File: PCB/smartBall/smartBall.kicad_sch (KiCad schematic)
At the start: 9 parts, among them IC12 ADM7155ACPZ-04-R7, IC3 ESP32-S3-WROOM-1-N4R8

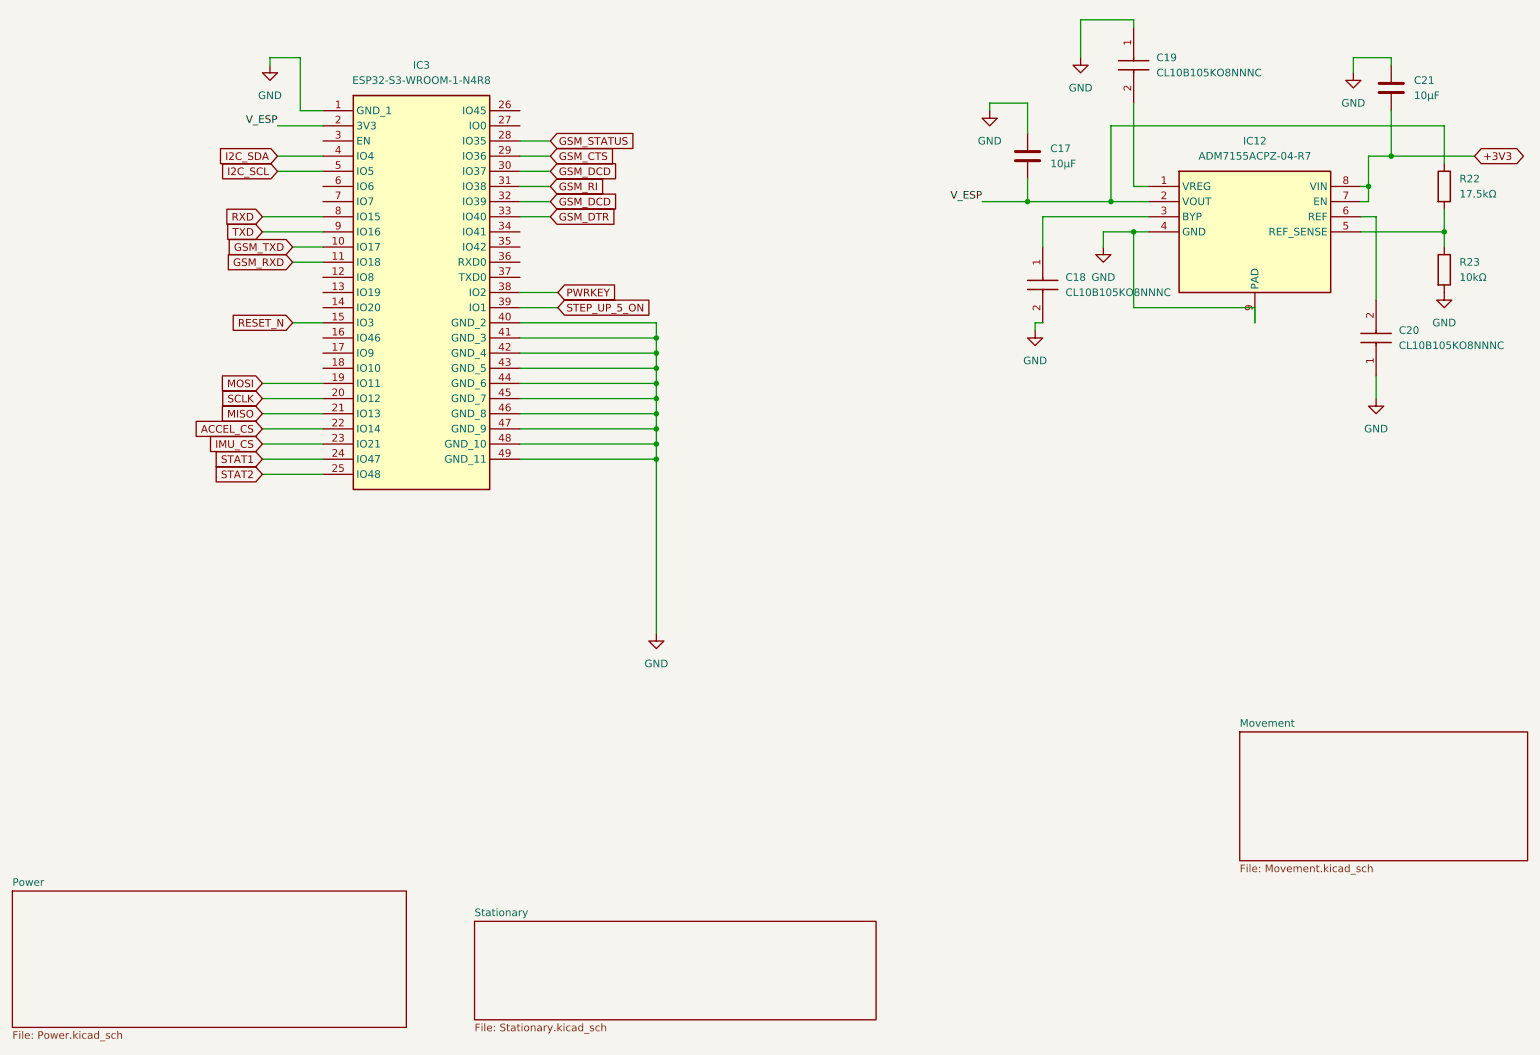
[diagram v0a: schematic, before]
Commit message: schematic ready
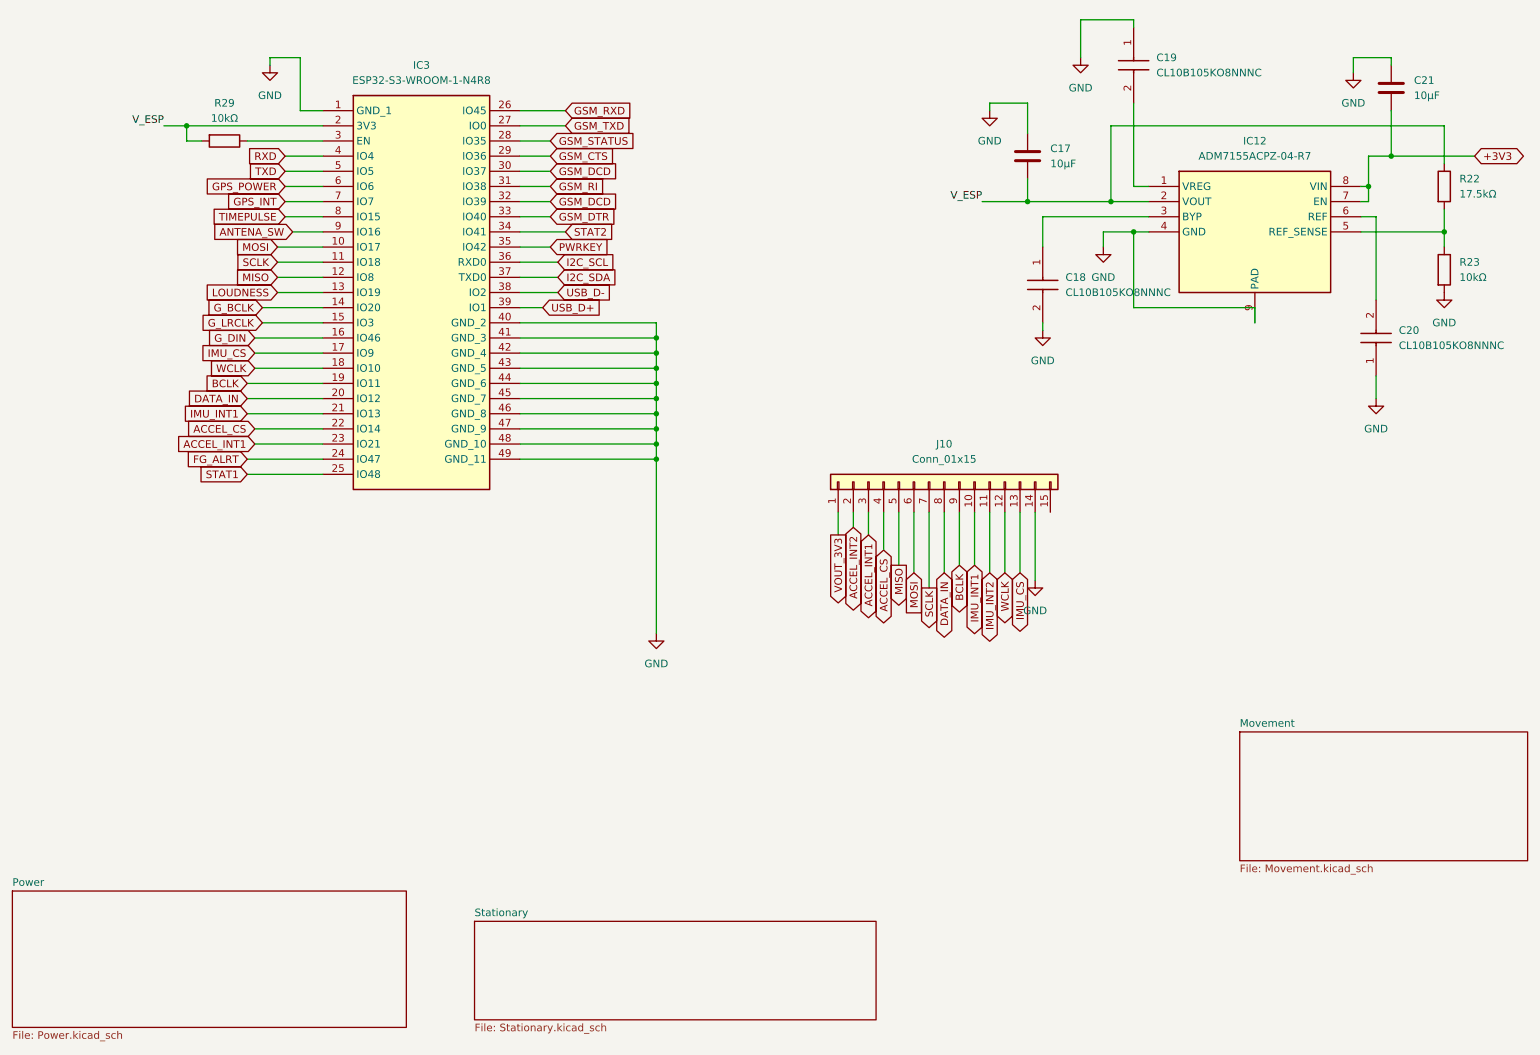
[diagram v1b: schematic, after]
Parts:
- added J10: Conn_01x15, symbol Connector_Generic:Conn_01x15
- added R29: 10kΩ, symbol Device:R
- IC12: footprint SON50P300X300X80-9N-D -> ADM7155ACPZ-04-07:SON50P300X300X80-9N-D
- IC3: footprint ESP32S3WROOM1N4R8 -> ESP_32-S3-WROOM-1-N4R8:ESP32S3WROOM1N4R8
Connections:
- net ACCEL_CS: now also J10.4 (Pin_4)
- net GND: now also J10.14 (Pin_14)
- net GSM_RXD: now also IC3.26 (IO45); no longer IC3.11 (IO18)
- net GSM_TXD: now also IC3.27 (IO0); no longer IC3.10 (IO17)
- net I2C_SCL: now also IC3.36 (RXD0); no longer IC3.5 (IO5)
- net I2C_SDA: now also IC3.37 (TXD0); no longer IC3.4 (IO4)
- net IMU_CS: now also IC3.17 (IO9), J10.13 (Pin_13); no longer IC3.23 (IO21)
- net MISO: now also IC3.12 (IO8), J10.5 (Pin_5); no longer IC3.21 (IO13)
- net MOSI: now also IC3.10 (IO17), J10.6 (Pin_6); no longer IC3.19 (IO11)
- net PWRKEY: now also IC3.35 (IO42); no longer IC3.38 (IO2)
- net RXD: now also IC3.4 (IO4); no longer IC3.8 (IO15)
- net SCLK: now also IC3.11 (IO18), J10.7 (Pin_7); no longer IC3.20 (IO12)
- net STAT1: now also IC3.25 (IO48); no longer IC3.24 (IO47)
- net STAT2: now also IC3.34 (IO41); no longer IC3.25 (IO48)
- net TXD: now also IC3.5 (IO5); no longer IC3.9 (IO16)
- net V_ESP: now also R29.2
- net LOUDNESS: now reaches IC3.13 (IO19)
- net G_BCLK: now reaches IC3.14 (IO20)
- net G_DIN: now reaches IC3.16 (IO46)
- net WCLK: now reaches IC3.18 (IO10)
- net WCLK: now also J10.12 (Pin_12)
- net at IC3.3 (EN): now also R29.1
- net GPS_POWER: now reaches IC3.6 (IO6)
- net GPS_INT: now reaches IC3.7 (IO7)
- net RESET_N renamed G_LRCLK
- net STEP_UP_5_ON renamed USB_D+
- new net ACCEL_INT1: IC3.23 (IO21), J10.3 (Pin_3)
- new net ACCEL_INT2: J10.2 (Pin_2)
- new net ANTENA_SW: IC3.9 (IO16)
- new net BCLK: IC3.19 (IO11), J10.9 (Pin_9)
- new net DATA_IN: IC3.20 (IO12), J10.8 (Pin_8)
- new net FG_ALRT: IC3.24 (IO47)
- new net IMU_INT1: IC3.21 (IO13), J10.10 (Pin_10)
- new net IMU_INT2: J10.11 (Pin_11)
- new net TIMEPULSE: IC3.8 (IO15)
- new net USB_D-: IC3.38 (IO2)
- new net VOUT_3V3: J10.1 (Pin_1)

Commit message: footprints assigned
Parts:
- C17, C21: footprint (none) -> Capacitor_THT:CP_Radial_Tantal_D5.0mm_P2.50mm
- C18, C19, C20: footprint CAPC1608X90N -> CL10B105KO8NNNC:CAPC1608X90N
- J10: footprint (none) -> Connector_PinHeader_2.54mm:PinHeader_1x15_P2.54mm_Vertical
- R22, R23, R29: footprint (none) -> Resistor_THT:R_Axial_DIN0207_L6.3mm_D2.5mm_P7.62mm_Horizontal
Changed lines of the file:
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@@
 			)
 		)
-		(property "Footprint" "CAPC1608X90N"
+		(property "Footprint" "CL10B105KO8NNNC:CAPC1608X90N"
 			(at 343.84 68.58 0)
 			(effects
@@
 			)
 		)
-		(property "Footprint" ""
+		(property "Footprint" "Resistor_THT:R_Axial_DIN0207_L6.3mm_D2.5mm_P7.62mm_Horizontal"
 			(at 257.302 59.69 90)
 			(effects
@@
 			)
 		)
-		(property "Footprint" ""
+		(property "Footprint" "Capacitor_THT:CP_Radial_Tantal_D5.0mm_P2.50mm"
 			(at 251.1552 33.02 0)
 			(effects
@@
 			)
 		)
-		(property "Footprint" "CAPC1608X90N"
+		(property "Footprint" "CL10B105KO8NNNC:CAPC1608X90N"
 			(at 95.58 64.77 0)
 			(effects
@@
 			)
 		)
-		(property "Footprint" ""
+		(property "Footprint" "Resistor_THT:R_Axial_DIN0207_L6.3mm_D2.5mm_P7.62mm_Horizontal"
 			(at 257.302 45.72 90)
 			(effects
@@
 			)
 		)
-		(property "Footprint" ""
+		(property "Footprint" "Connector_PinHeader_2.54mm:PinHeader_1x15_P2.54mm_Vertical"
 			(at 175.26 95.25 0)
 			(effects
@@
 			)
 		)
-		(property "Footprint" ""
+		(property "Footprint" "Capacitor_THT:CP_Radial_Tantal_D5.0mm_P2.50mm"
 			(at 190.1952 44.45 0)
 			(effects
@@
 			)
 		)
-		(property "Footprint" "CAPC1608X90N"
+		(property "Footprint" "CL10B105KO8NNNC:CAPC1608X90N"
 			(at 110.82 27.94 0)
 			(effects
@@
 			)
 		)
-		(property "Footprint" ""
+		(property "Footprint" "Resistor_THT:R_Axial_DIN0207_L6.3mm_D2.5mm_P7.62mm_Horizontal"
 			(at 54.61 36.322 90)
 			(effects

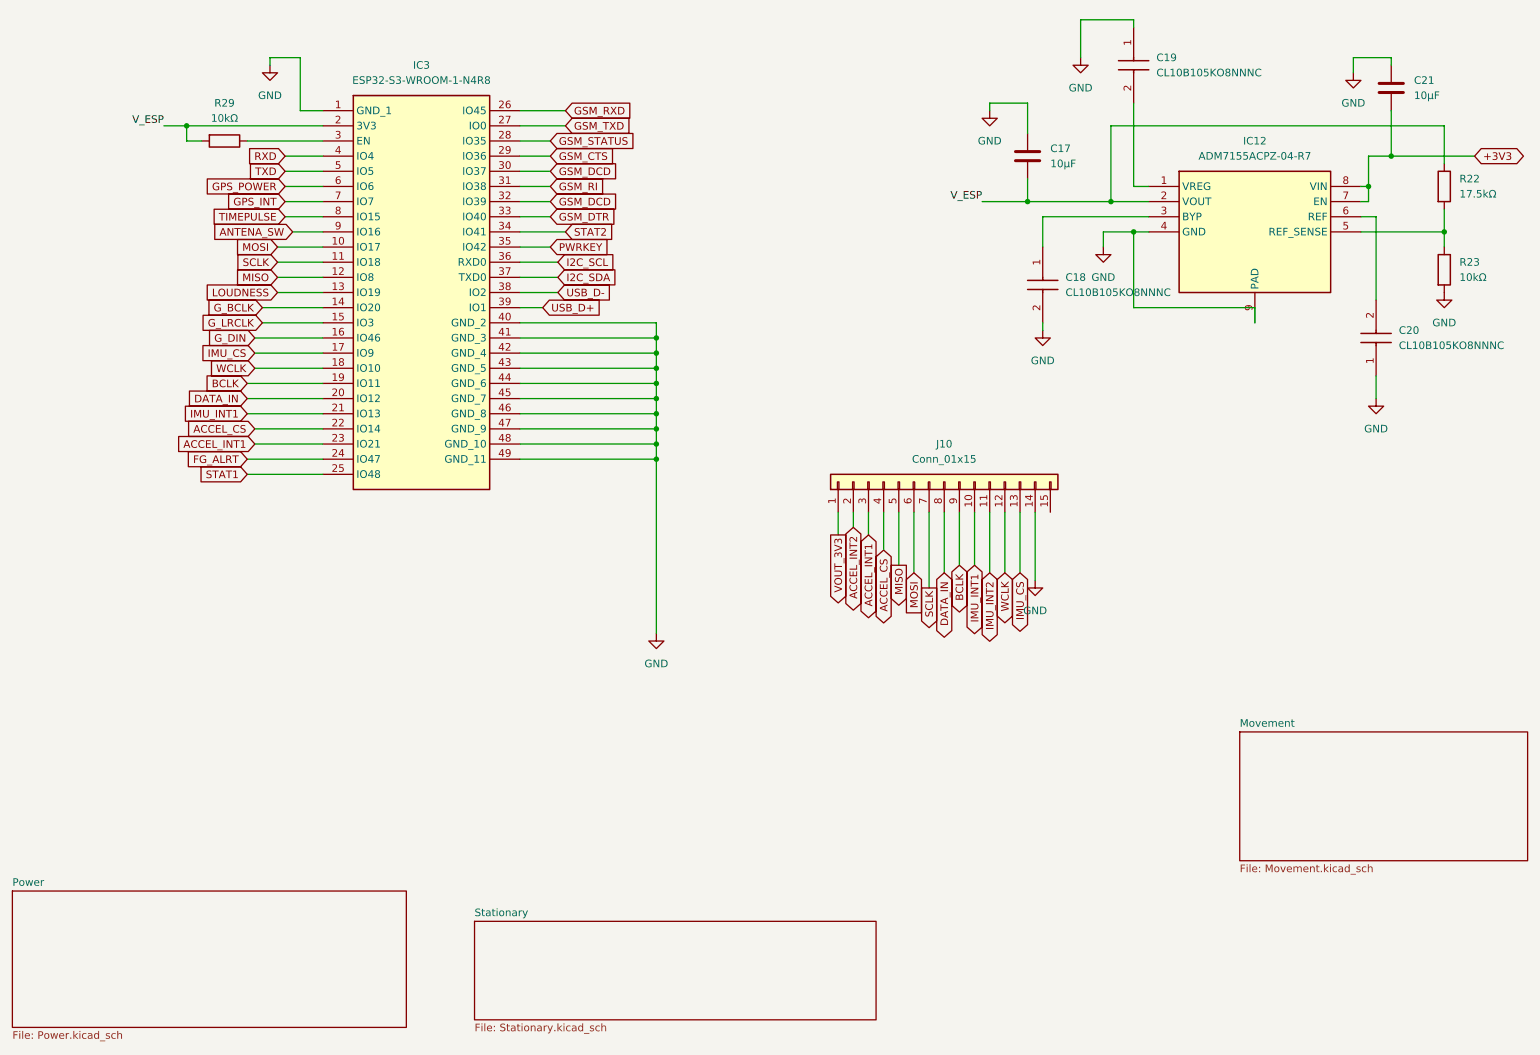
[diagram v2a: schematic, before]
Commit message: updated to hierarchical labels
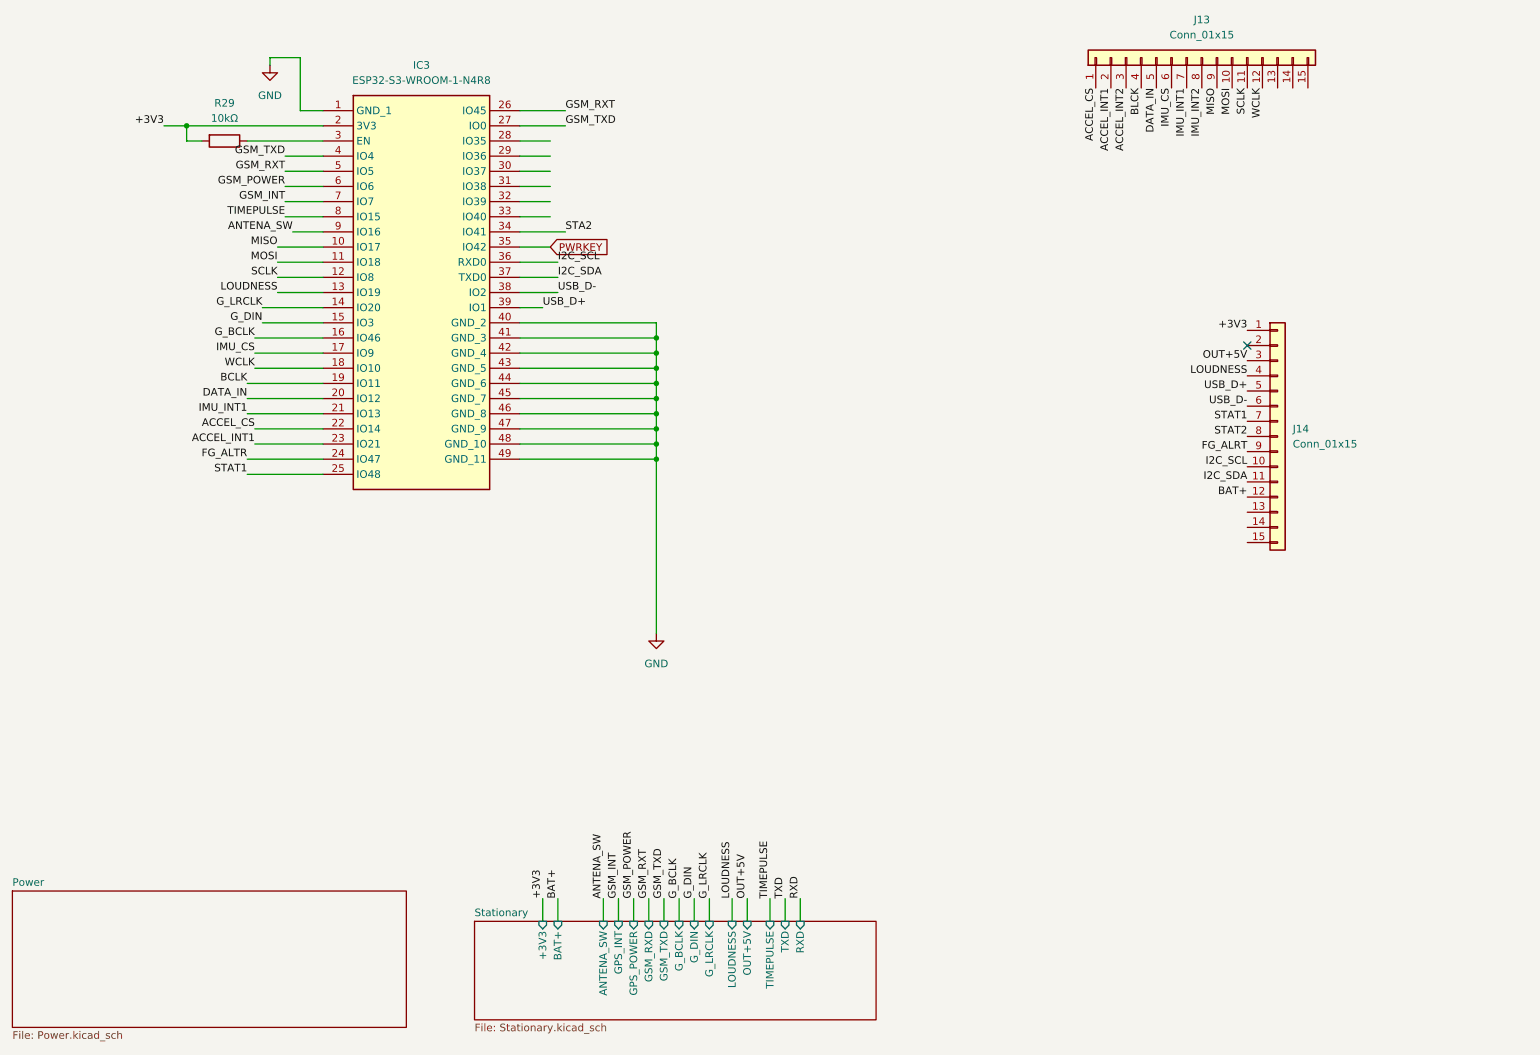
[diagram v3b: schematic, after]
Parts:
- removed C17, C21: 10µF, Capacitor_THT:CP_Radial_Tantal_D5.0mm_P2.50mm, symbol Device:C
- removed C18, C19, C20: CL10B105KO8NNNC, CL10B105KO8NNNC:CAPC1608X90N, symbol CL10B105KO8NNNC:CL10B105KO8NNNC
- removed IC12: ADM7155ACPZ-04-R7, ADM7155ACPZ-04-07:SON50P300X300X80-9N-D, symbol ADM7155ACPZ-04-R7:ADM7155ACPZ-04-R7
- removed J10: Conn_01x15, Connector_PinHeader_2.54mm:PinHeader_1x15_P2.54mm_Vertical, symbol Connector_Generic:Conn_01x15
- removed R22: 17.5kΩ, Resistor_THT:R_Axial_DIN0207_L6.3mm_D2.5mm_P7.62mm_Horizontal, symbol Device:R
- removed R23: 10kΩ, Resistor_THT:R_Axial_DIN0207_L6.3mm_D2.5mm_P7.62mm_Horizontal, symbol Device:R
- added J13, J14: Conn_01x15, Connector_PinHeader_2.54mm:PinHeader_1x15_P2.54mm_Vertical, symbol Connector_Generic:Conn_01x15
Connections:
- net V_ESP is gone; now on net +3V3: IC3.2 (3V3), R29.2
- net +3V3: now also J14.1 (Pin_1)
- net ACCEL_CS: now also J13.1 (Pin_1)
- net ACCEL_INT1: now also J13.2 (Pin_2)
- net ACCEL_INT2: now also J13.3 (Pin_3)
- net DATA_IN: now also J13.5 (Pin_5)
- net FG_ALRT: now also J14.9 (Pin_9); no longer IC3.24 (IO47)
- net GSM_TXD: now also IC3.4 (IO4)
- net G_BCLK: now also IC3.16 (IO46); no longer IC3.14 (IO20)
- net G_DIN: now also IC3.15 (IO3); no longer IC3.16 (IO46)
- net G_LRCLK: now also IC3.14 (IO20); no longer IC3.15 (IO3)
- net I2C_SCL: now also J14.10 (Pin_10)
- net I2C_SDA: now also J14.11 (Pin_11)
- net IMU_CS: now also J13.6 (Pin_6)
- net IMU_INT1: now also J13.7 (Pin_7)
- net IMU_INT2: now also J13.8 (Pin_8)
- net LOUDNESS: now also J14.4 (Pin_4)
- net MISO: now also IC3.10 (IO17), J13.9 (Pin_9); no longer IC3.12 (IO8)
- net MOSI: now also IC3.11 (IO18), J13.10 (Pin_10); no longer IC3.10 (IO17)
- net RXD: no longer IC3.4 (IO4)
- net SCLK: now also IC3.12 (IO8), J13.11 (Pin_11); no longer IC3.11 (IO18)
- net STAT1: now also J14.7 (Pin_7)
- net STAT2: now also J14.8 (Pin_8); no longer IC3.34 (IO41)
- net TXD: no longer IC3.5 (IO5)
- net USB_D+: now also J14.5 (Pin_5)
- net USB_D-: now also J14.6 (Pin_6)
- net WCLK: now also J13.12 (Pin_12)
- net GPS_INT renamed GSM_INT
- net GPS_POWER renamed GSM_POWER
- net GSM_CTS: no longer names the net of IC3.29 (IO36)
- net GSM_DCD: no longer names the net of IC3.30 (IO37)
- net GSM_DCD: no longer IC3.32 (IO39)
- net GSM_DTR: no longer names the net of IC3.33 (IO40)
- net GSM_RI: no longer names the net of IC3.31 (IO38)
- net GSM_RXD renamed GSM_RXT
- net GSM_RXT: now also IC3.5 (IO5)
- net GSM_STATUS: no longer names the net of IC3.28 (IO35)
- new net BAT+: J14.12 (Pin_12)
- new net BLCK: J13.4 (Pin_4)
- new net FG_ALTR: IC3.24 (IO47)
- new net OUT+5V: J14.3 (Pin_3)
- new net STA2: IC3.34 (IO41)
- no-connect marks 0 -> 1
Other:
- removed sheet Movement
- sheet Stationary ports: added +3V3, ANTENA_SW, BAT+, GPS_INT, GPS_POWER, GSM_RXD, GSM_TXD, G_BCLK, G_DIN, G_LRCLK, LOUDNESS, OUT+5V, RXD, TIMEPULSE, TXD; removed none
